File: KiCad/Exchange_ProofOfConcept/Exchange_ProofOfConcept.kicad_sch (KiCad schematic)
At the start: 29 parts, among them J1 Conn_02x03_Odd_Even, J2 Conn_02x03_Odd_Even, J3 Conn_01x07, J7 Screw_Terminal_01x02, J9 Screw_Terminal_01x08, U1 MCP23017, U2 MCP23017, U3 MT8816

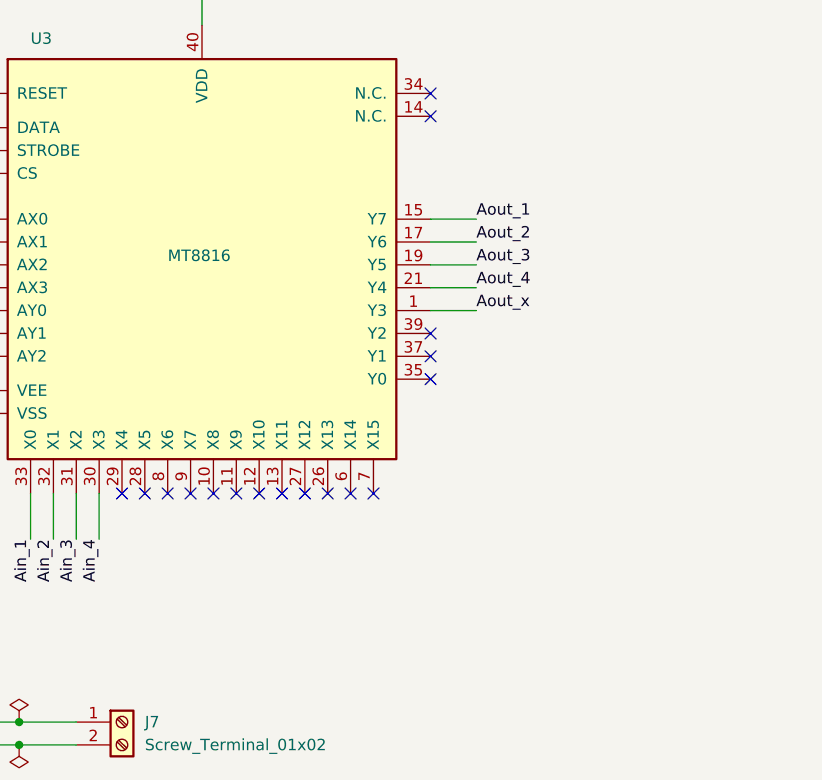
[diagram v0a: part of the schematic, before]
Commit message: deleted:    KiCad/Exchange_ProofOfConcept/#auto_saved_files# 	deleted:    KiCad/Exchange_ProofOfConcept/Exchange_ProofOfConcept-backups/Exchange_ProofOfConcept-2024-11-26_195718.zip 	new file:   KiCad/Exchange_ProofOfConcept/Exchange_ProofOfConcept-backups/Exchange_ProofOfConcept-2025-02-02_182812.zip 	modified:   KiCad/Exchange_ProofOfConcept/Exchange_ProofOfConcept.kicad_sch 	modified:   KiCad/Exchange_ProofOfConcept/SLIC 1.kicad_sch 	modified:   KiCad/Exchange_ProofOfConcept/SLIC 1_sch.kicad_sch 	modified:   KiCad/Exchange_ProofOfConcept/SLIC 3.kicad_sch 	modified:   KiCad/Exchange_ProofOfConcept/SLIC 4.kicad_sch 	deleted:    KiCad/Exchange_ProofOfConcept/_autosave-Exchange_ProofOfConcept.kicad_sch 	deleted:    KiCad/Exchange_ProofOfConcept/~Exchange_ProofOfConcept.kicad_pcb.lck 	deleted:    KiCad/Exchange_ProofOfConcept/~Exchange_ProofOfConcept.kicad_sch.lck 	modified:   docs/European harmonization of network generated tones.pdf 	modified:   include/config.h 	modified:   platformio.ini
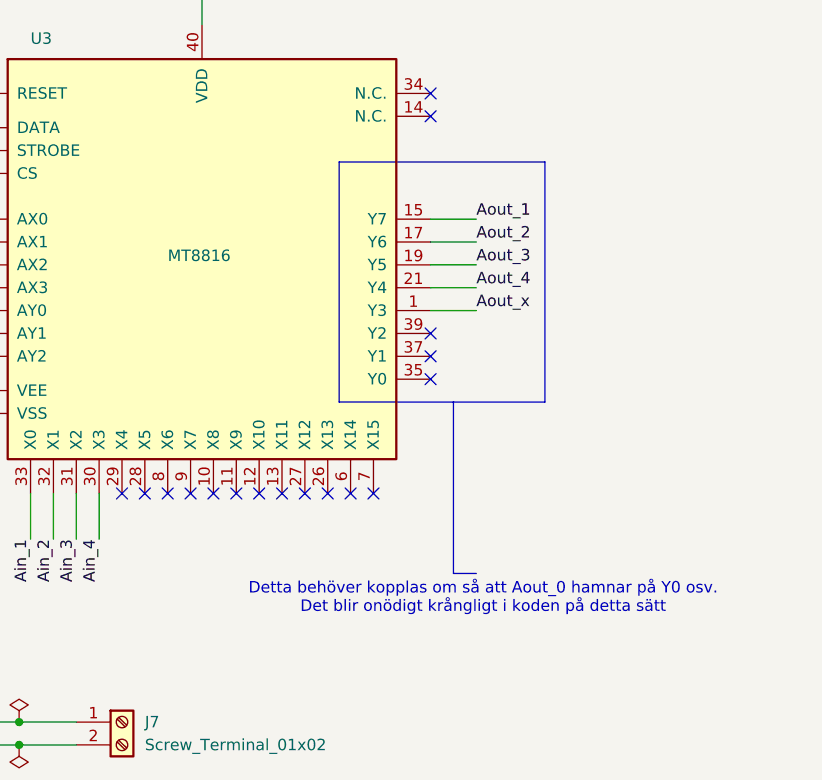
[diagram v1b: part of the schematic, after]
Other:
- note added: "Detta behöver kopplas om så att Aout_0 hamnar på Y0 osv. Det blir onödigt krångligt i koden på detta sätt"
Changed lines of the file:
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@@
+		)
+	)
+	(polyline
+		(pts
+			(xy 273.05 73.66) (xy 273.05 92.71)
+		)
+		(stroke
+			(width 0)
+			(type default)
 		)
 	)
@@
 		)
 	)
+	(polyline
+		(pts
+			(xy 273.05 92.71) (xy 275.59 92.71)
+		)
+		(stroke
+			(width 0)
+			(type default)
+		)
+	)
 	(wire
 		(pts
@@
 			(width 0)
 			(type default)
+		)
+	)
+	(rectangle
+		(start 260.35 46.99)
+		(end 283.21 73.66)
+		(stroke
+			(width 0)
+			(type default)
+		)
+		(fill
+			(type none)
 		)
 	)
@@
 		)
 	)
+	(text "Detta behöver kopplas om så att Aout_0 hamnar på Y0 osv. \nDet blir onödigt krångligt i koden på detta sätt\n"
+		(exclude_from_sim no)
+		(at 276.352 95.504 0)
+		(effects
+			(font
+				(size 1.27 1.27)
+			)
+		)
+	)
 	(label "Ain_3"
 		(at 87.63 81.28 180)
-		(fields_autoplaced yes)
 		(effects
 			(font
@@
 	(label "Aout_x"
 		(at 275.59 63.5 0)
-		(fields_autoplaced yes)
 		(effects
 			(font
@@
 	(label "5V"
 		(at 17.78 143.51 0)
-		(fields_autoplaced yes)
 		(effects
 			(font
@@
 	(label "Aout_1"
 		(at 275.59 53.34 0)
-		(fields_autoplaced yes)
 		(effects
 			(font
@@
 	(label "Aout_1"
 		(at 45.72 34.29 0)
-		(fields_autoplaced yes)
 		(effects
 			(font
@@
 	(label "RING_2"
 		(at 45.72 69.85 0)
-		(fields_autoplaced yes)
 		(effects
 			(font
@@
 	(label "5V"
 		(at 171.45 21.59 0)
-		(fields_autoplaced yes)
 		(effects
 			(font
@@
 	(label "SCL"
 		(at 194.31 121.92 180)
-		(fields_autoplaced yes)
 		(effects
 			(font
@@
 	(label "5V"
 		(at 36.83 187.96 180)
-		(fields_autoplaced yes)
 		(effects
 			(font
@@
 	(label "Ain_2"
 		(at 228.6 88.9 270)
-		(fields_autoplaced yes)
 		(effects
 			(font
@@
 	(label "Aout_3"
 		(at 275.59 58.42 0)
-		(fields_autoplaced yes)
 		(effects
 			(font
@@
 	(label "RING_4"
 		(at 223.52 146.05 180)
-		(fields_autoplaced yes)
 		(effects
 			(font
@@
 	(label "Aout_3"
 		(at 87.63 78.74 180)
-		(fields_autoplaced yes)
 		(effects
 			(font
@@
 	(label "RING_3"
 		(at 87.63 72.39 180)
-		(fields_autoplaced yes)
 		(effects
 			(font
@@
 	(label "SDA"
 		(at 194.31 119.38 180)
-		(fields_autoplaced yes)
 		(effects
 			(font
@@
 	(label "TIP_4"
 		(at 223.52 143.51 180)
-		(fields_autoplaced yes)
 		(effects
 			(font
@@
 	(label "TIP_4"
 		(at 85.09 27.94 180)
-		(fields_autoplaced yes)
 		(effects
 			(font
@@
 	(label "Aout_2"
 		(at 275.59 55.88 0)
-		(fields_autoplaced yes)
 		(effects
 			(font
@@
 	(label "TIP_3"
 		(at 223.52 148.59 180)
-		(fields_autoplaced yes)
 		(effects
 			(font
@@
 	(label "RING_3"
 		(at 223.52 151.13 180)
-		(fields_autoplaced yes)
 		(effects
 			(font
@@
 	(label "Ain_1"
 		(at 226.06 88.9 270)
-		(fields_autoplaced yes)
 		(effects
 			(font
@@
 	(label "Aout_x"
 		(at 222.25 129.54 180)
-		(fields_autoplaced yes)
 		(effects
 			(font
@@
 	(label "5V"
 		(at 21.59 60.96 0)
-		(fields_autoplaced yes)
 		(effects
 			(font
@@
 	(label "Aout_4"
 		(at 85.09 34.29 180)
-		(fields_autoplaced yes)
 		(effects
 			(font
@@
 	(label "SLIC_INT"
 		(at 99.06 111.76 0)
-		(fields_autoplaced yes)
 		(effects
 			(font
@@
 	(label "Aout_4"
 		(at 275.59 60.96 0)
-		(fields_autoplaced yes)
 		(effects
 			(font
@@
 	(label "5V"
 		(at 107.95 60.96 0)
-		(fields_autoplaced yes)
 		(effects
 			(font
@@
 	(label "TIP_3"
 		(at 87.63 69.85 180)
-		(fields_autoplaced yes)
 		(effects
 			(font
@@
 	(label "SCL"
 		(at 139.7 78.74 180)
-		(fields_autoplaced yes)
 		(effects
 			(font
@@
 	(label "MCP_reset"
 		(at 222.25 127 180)
-		(fields_autoplaced yes)
 		(effects
 			(font
@@
 	(label "5V"
 		(at 222.25 132.08 180)
-		(fields_autoplaced yes)
 		(effects
 			(font
@@
 	(label "RING_2"
 		(at 223.52 156.21 180)
-		(fields_autoplaced yes)
 		(effects
 			(font
@@
 	(label "TIP_1"
 		(at 45.72 27.94 0)
-		(fields_autoplaced yes)
 		(effects
 			(font
@@
 	(label "TIP_1"
 		(at 223.52 158.75 180)
-		(fields_autoplaced yes)
 		(effects
 			(font
@@
 	(label "MCP_reset"
 		(at 135.89 30.48 90)
-		(fields_autoplaced yes)
 		(effects
 			(font
@@
 	(label "Aout_2"
 		(at 45.72 78.74 0)
-		(fields_autoplaced yes)
 		(effects
 			(font
@@
 	(label "5V"
 		(at 127 30.48 180)
-		(fields_autoplaced yes)
 		(effects
 			(font
@@
 	(label "RING_1"
 		(at 223.52 161.29 180)
-		(fields_autoplaced yes)
 		(effects
 			(font
@@
 	(label "Ain_4"
 		(at 85.09 36.83 180)
-		(fields_autoplaced yes)
 		(effects
 			(font
@@
 	(label "TIP_2"
 		(at 45.72 72.39 0)
-		(fields_autoplaced yes)
 		(effects
 			(font
@@
 	(label "MCP_reset"
 		(at 36.83 179.07 180)
-		(fields_autoplaced yes)
 		(effects
 			(font
@@
 	(label "Ain_4"
 		(at 233.68 88.9 270)
-		(fields_autoplaced yes)
 		(effects
 			(font
@@
 	(label "Ain_2"
 		(at 45.72 81.28 0)
-		(fields_autoplaced yes)
 		(effects
 			(font
@@
 	(label "Ain_1"
 		(at 45.72 36.83 0)
-		(fields_autoplaced yes)
 		(effects
 			(font
@@
 	(label "5V"
 		(at 27.94 16.51 0)
-		(fields_autoplaced yes)
 		(effects
 			(font
@@
 	(label "Ain_3"
 		(at 231.14 88.9 270)
-		(fields_autoplaced yes)
 		(effects
 			(font
@@
 	(label "5V"
 		(at 165.1 106.68 180)
-		(fields_autoplaced yes)
 		(effects
 			(font
@@
 	(label "RING_1"
 		(at 45.72 25.4 0)
-		(fields_autoplaced yes)
 		(effects
 			(font
@@
 	(label "5V"
 		(at 102.87 16.51 0)
-		(fields_autoplaced yes)
 		(effects
 			(font
@@
 	(label "5V"
 		(at 205.74 153.67 180)
-		(fields_autoplaced yes)
 		(effects
 			(font
@@
 	(label "SDA"
 		(at 82.55 171.45 270)
-		(fields_autoplaced yes)
 		(effects
 			(font
@@
 	(label "RING_4"
 		(at 85.09 25.4 180)
-		(fields_autoplaced yes)
 		(effects
 			(font
@@
 	(label "SDA"
 		(at 139.7 76.2 180)
-		(fields_autoplaced yes)
 		(effects
 			(font
@@
 	(label "SLIC_INT"
 		(at 222.25 124.46 180)
-		(fields_autoplaced yes)
 		(effects
 			(font
@@
 	(label "SCL"
 		(at 85.09 171.45 270)
-		(fields_autoplaced yes)
 		(effects
 			(font
@@
 	(label "5V"
 		(at 245.11 26.67 0)
-		(fields_autoplaced yes)
 		(effects
 			(font
@@
 	(label "TIP_2"
 		(at 223.52 153.67 180)
-		(fields_autoplaced yes)
 		(effects
 			(font
@@
 	(label "GND"
 		(at 165.1 111.76 180)
-		(fields_autoplaced yes)
-		(effects
-			(font
+		(effects
+			(font

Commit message: Revert "Number dailing"
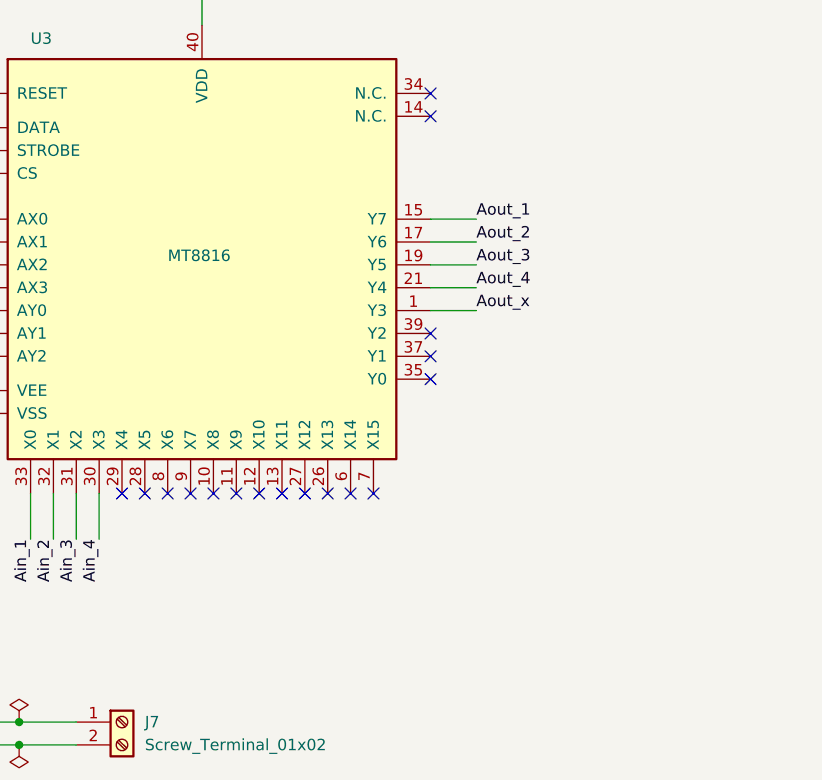
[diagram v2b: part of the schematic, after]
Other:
- note removed: "Detta behöver kopplas om så att Aout_0 hamnar på Y0 osv. Det blir onödigt krångligt i koden på detta sätt"
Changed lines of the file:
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@@
-		)
-	)
-	(polyline
-		(pts
-			(xy 273.05 73.66) (xy 273.05 92.71)
-		)
-		(stroke
-			(width 0)
-			(type default)
 		)
 	)
@@
 		)
 	)
-	(polyline
-		(pts
-			(xy 273.05 92.71) (xy 275.59 92.71)
-		)
-		(stroke
-			(width 0)
-			(type default)
-		)
-	)
 	(wire
 		(pts
@@
 			(width 0)
 			(type default)
-		)
-	)
-	(rectangle
-		(start 260.35 46.99)
-		(end 283.21 73.66)
-		(stroke
-			(width 0)
-			(type default)
-		)
-		(fill
-			(type none)
 		)
 	)
@@
 		)
 	)
-	(text "Detta behöver kopplas om så att Aout_0 hamnar på Y0 osv. \nDet blir onödigt krångligt i koden på detta sätt\n"
-		(exclude_from_sim no)
-		(at 276.352 95.504 0)
-		(effects
-			(font
-				(size 1.27 1.27)
-			)
-		)
-	)
 	(label "Ain_3"
 		(at 87.63 81.28 180)
+		(fields_autoplaced yes)
 		(effects
 			(font
@@
 	(label "Aout_x"
 		(at 275.59 63.5 0)
+		(fields_autoplaced yes)
 		(effects
 			(font
@@
 	(label "5V"
 		(at 17.78 143.51 0)
+		(fields_autoplaced yes)
 		(effects
 			(font
@@
 	(label "Aout_1"
 		(at 275.59 53.34 0)
+		(fields_autoplaced yes)
 		(effects
 			(font
@@
 	(label "Aout_1"
 		(at 45.72 34.29 0)
+		(fields_autoplaced yes)
 		(effects
 			(font
@@
 	(label "RING_2"
 		(at 45.72 69.85 0)
+		(fields_autoplaced yes)
 		(effects
 			(font
@@
 	(label "5V"
 		(at 171.45 21.59 0)
+		(fields_autoplaced yes)
 		(effects
 			(font
@@
 	(label "SCL"
 		(at 194.31 121.92 180)
+		(fields_autoplaced yes)
 		(effects
 			(font
@@
 	(label "5V"
 		(at 36.83 187.96 180)
+		(fields_autoplaced yes)
 		(effects
 			(font
@@
 	(label "Ain_2"
 		(at 228.6 88.9 270)
+		(fields_autoplaced yes)
 		(effects
 			(font
@@
 	(label "Aout_3"
 		(at 275.59 58.42 0)
+		(fields_autoplaced yes)
 		(effects
 			(font
@@
 	(label "RING_4"
 		(at 223.52 146.05 180)
+		(fields_autoplaced yes)
 		(effects
 			(font
@@
 	(label "Aout_3"
 		(at 87.63 78.74 180)
+		(fields_autoplaced yes)
 		(effects
 			(font
@@
 	(label "RING_3"
 		(at 87.63 72.39 180)
+		(fields_autoplaced yes)
 		(effects
 			(font
@@
 	(label "SDA"
 		(at 194.31 119.38 180)
+		(fields_autoplaced yes)
 		(effects
 			(font
@@
 	(label "TIP_4"
 		(at 223.52 143.51 180)
+		(fields_autoplaced yes)
 		(effects
 			(font
@@
 	(label "TIP_4"
 		(at 85.09 27.94 180)
+		(fields_autoplaced yes)
 		(effects
 			(font
@@
 	(label "Aout_2"
 		(at 275.59 55.88 0)
+		(fields_autoplaced yes)
 		(effects
 			(font
@@
 	(label "TIP_3"
 		(at 223.52 148.59 180)
+		(fields_autoplaced yes)
 		(effects
 			(font
@@
 	(label "RING_3"
 		(at 223.52 151.13 180)
+		(fields_autoplaced yes)
 		(effects
 			(font
@@
 	(label "Ain_1"
 		(at 226.06 88.9 270)
+		(fields_autoplaced yes)
 		(effects
 			(font
@@
 	(label "Aout_x"
 		(at 222.25 129.54 180)
+		(fields_autoplaced yes)
 		(effects
 			(font
@@
 	(label "5V"
 		(at 21.59 60.96 0)
+		(fields_autoplaced yes)
 		(effects
 			(font
@@
 	(label "Aout_4"
 		(at 85.09 34.29 180)
+		(fields_autoplaced yes)
 		(effects
 			(font
@@
 	(label "SLIC_INT"
 		(at 99.06 111.76 0)
+		(fields_autoplaced yes)
 		(effects
 			(font
@@
 	(label "Aout_4"
 		(at 275.59 60.96 0)
+		(fields_autoplaced yes)
 		(effects
 			(font
@@
 	(label "5V"
 		(at 107.95 60.96 0)
+		(fields_autoplaced yes)
 		(effects
 			(font
@@
 	(label "TIP_3"
 		(at 87.63 69.85 180)
+		(fields_autoplaced yes)
 		(effects
 			(font
@@
 	(label "SCL"
 		(at 139.7 78.74 180)
+		(fields_autoplaced yes)
 		(effects
 			(font
@@
 	(label "MCP_reset"
 		(at 222.25 127 180)
+		(fields_autoplaced yes)
 		(effects
 			(font
@@
 	(label "5V"
 		(at 222.25 132.08 180)
+		(fields_autoplaced yes)
 		(effects
 			(font
@@
 	(label "RING_2"
 		(at 223.52 156.21 180)
+		(fields_autoplaced yes)
 		(effects
 			(font
@@
 	(label "TIP_1"
 		(at 45.72 27.94 0)
+		(fields_autoplaced yes)
 		(effects
 			(font
@@
 	(label "TIP_1"
 		(at 223.52 158.75 180)
+		(fields_autoplaced yes)
 		(effects
 			(font
@@
 	(label "MCP_reset"
 		(at 135.89 30.48 90)
+		(fields_autoplaced yes)
 		(effects
 			(font
@@
 	(label "Aout_2"
 		(at 45.72 78.74 0)
+		(fields_autoplaced yes)
 		(effects
 			(font
@@
 	(label "5V"
 		(at 127 30.48 180)
+		(fields_autoplaced yes)
 		(effects
 			(font
@@
 	(label "RING_1"
 		(at 223.52 161.29 180)
+		(fields_autoplaced yes)
 		(effects
 			(font
@@
 	(label "Ain_4"
 		(at 85.09 36.83 180)
+		(fields_autoplaced yes)
 		(effects
 			(font
@@
 	(label "TIP_2"
 		(at 45.72 72.39 0)
+		(fields_autoplaced yes)
 		(effects
 			(font
@@
 	(label "MCP_reset"
 		(at 36.83 179.07 180)
+		(fields_autoplaced yes)
 		(effects
 			(font
@@
 	(label "Ain_4"
 		(at 233.68 88.9 270)
+		(fields_autoplaced yes)
 		(effects
 			(font
@@
 	(label "Ain_2"
 		(at 45.72 81.28 0)
+		(fields_autoplaced yes)
 		(effects
 			(font
@@
 	(label "Ain_1"
 		(at 45.72 36.83 0)
+		(fields_autoplaced yes)
 		(effects
 			(font
@@
 	(label "5V"
 		(at 27.94 16.51 0)
+		(fields_autoplaced yes)
 		(effects
 			(font
@@
 	(label "Ain_3"
 		(at 231.14 88.9 270)
+		(fields_autoplaced yes)
 		(effects
 			(font
@@
 	(label "5V"
 		(at 165.1 106.68 180)
+		(fields_autoplaced yes)
 		(effects
 			(font
@@
 	(label "RING_1"
 		(at 45.72 25.4 0)
+		(fields_autoplaced yes)
 		(effects
 			(font
@@
 	(label "5V"
 		(at 102.87 16.51 0)
+		(fields_autoplaced yes)
 		(effects
 			(font
@@
 	(label "5V"
 		(at 205.74 153.67 180)
+		(fields_autoplaced yes)
 		(effects
 			(font
@@
 	(label "SDA"
 		(at 82.55 171.45 270)
+		(fields_autoplaced yes)
 		(effects
 			(font
@@
 	(label "RING_4"
 		(at 85.09 25.4 180)
+		(fields_autoplaced yes)
 		(effects
 			(font
@@
 	(label "SDA"
 		(at 139.7 76.2 180)
+		(fields_autoplaced yes)
 		(effects
 			(font
@@
 	(label "SLIC_INT"
 		(at 222.25 124.46 180)
+		(fields_autoplaced yes)
 		(effects
 			(font
@@
 	(label "SCL"
 		(at 85.09 171.45 270)
+		(fields_autoplaced yes)
 		(effects
 			(font
@@
 	(label "5V"
 		(at 245.11 26.67 0)
+		(fields_autoplaced yes)
 		(effects
 			(font
@@
 	(label "TIP_2"
 		(at 223.52 153.67 180)
+		(fields_autoplaced yes)
 		(effects
 			(font
@@
 	(label "GND"
 		(at 165.1 111.76 180)
-		(effects
-			(font
+		(fields_autoplaced yes)
+		(effects
+			(font
